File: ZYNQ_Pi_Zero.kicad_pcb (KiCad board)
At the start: 4 copper layers, 35 parts, among them Q501 2N7002, Q502 2N7002, Q503 2N7002, U101 xc7z010clg400, U201 MT41K256M16TW-107_P, U301 W25Q256FVEI, U501 TPD4E05U06DQA, U502 TPD4E05U06DQA

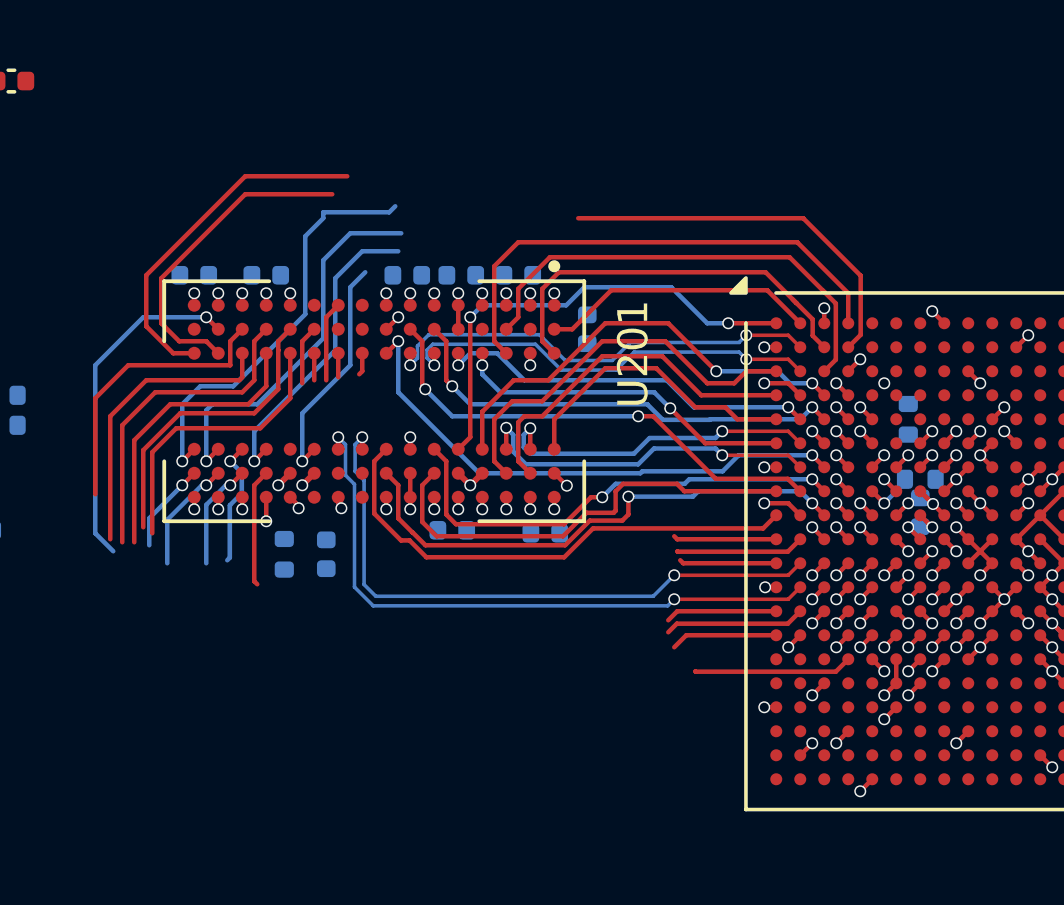
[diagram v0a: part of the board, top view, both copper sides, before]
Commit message: feat: continue routing ddr
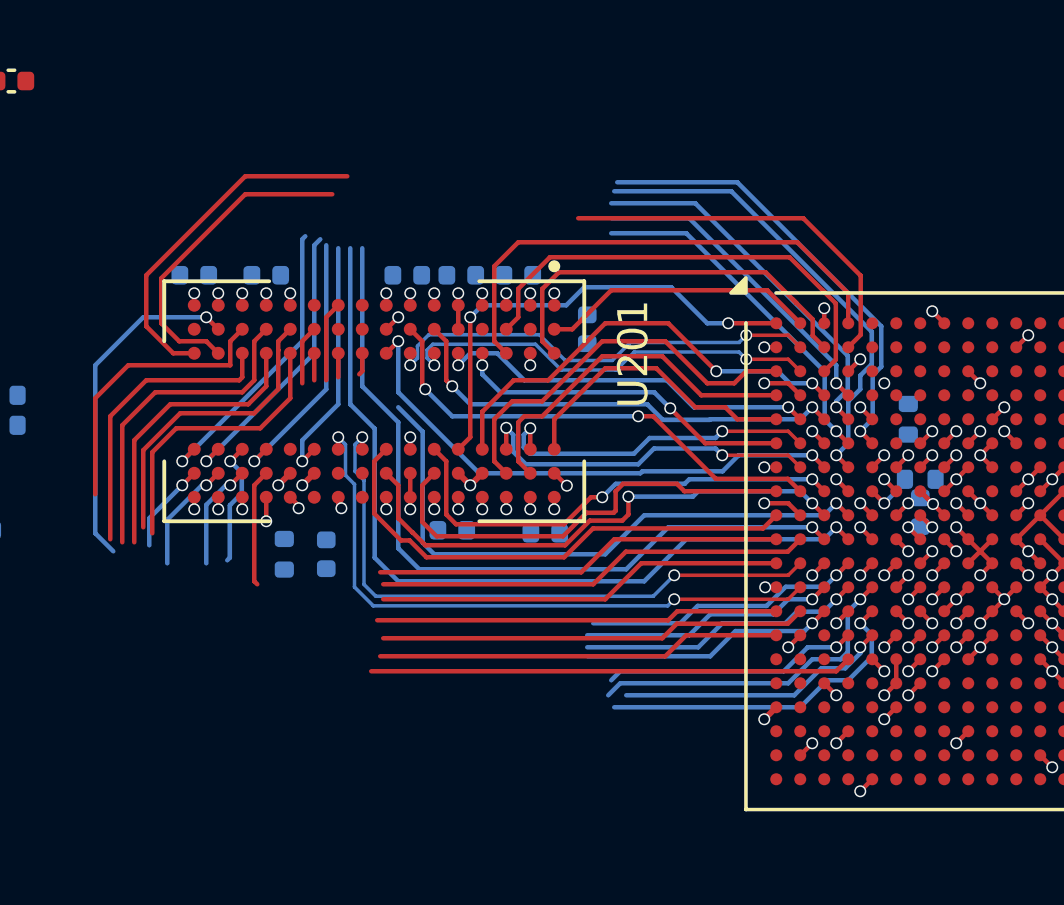
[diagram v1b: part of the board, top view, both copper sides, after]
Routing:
- net /DDR3/DDR_A7: track 11.9 -> 39.1 mm
- net /DDR3/DDR_A3: track 11.4 -> 36.5 mm
- net /DDR3/DDR_A9: track 11.2 -> 30.7 mm
- net /DDR3/DDR_A10: track 8.30 -> 23.3 mm
- net /DDR3/DDR_A11: track 13.3 -> 25.2 mm
- net /DDR3/DDR_BA1: track 9.18 -> 20.0 mm
- net /DDR3/DDR_ODT: track 3.23 -> 13.8 mm
- net /DDR3/DDR_~{WE}: track 1.47 -> 12.0 mm
- net /DDR3/DDR_A12: track 10.8 -> 21.2 mm
- net /DDR3/DDR_A5: track 12.8 -> 23.1 mm
- net /DDR3/DDR_A1: track 8.50 -> 18.7 mm
- net /DDR3/DDR_A8: track 6.46 -> 16.7 mm
- net /DDR3/DDR_A13: track 12.3 -> 22.4 mm
- net unconnected-(U101G-PS_DDR_DQ16_502-PadP1): track 3.57 -> 13.5 mm
- net /DDR3/DDR_~{CS}: track 5.69 -> 15.4 mm
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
